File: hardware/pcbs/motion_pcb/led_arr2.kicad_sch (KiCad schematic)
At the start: 21 parts

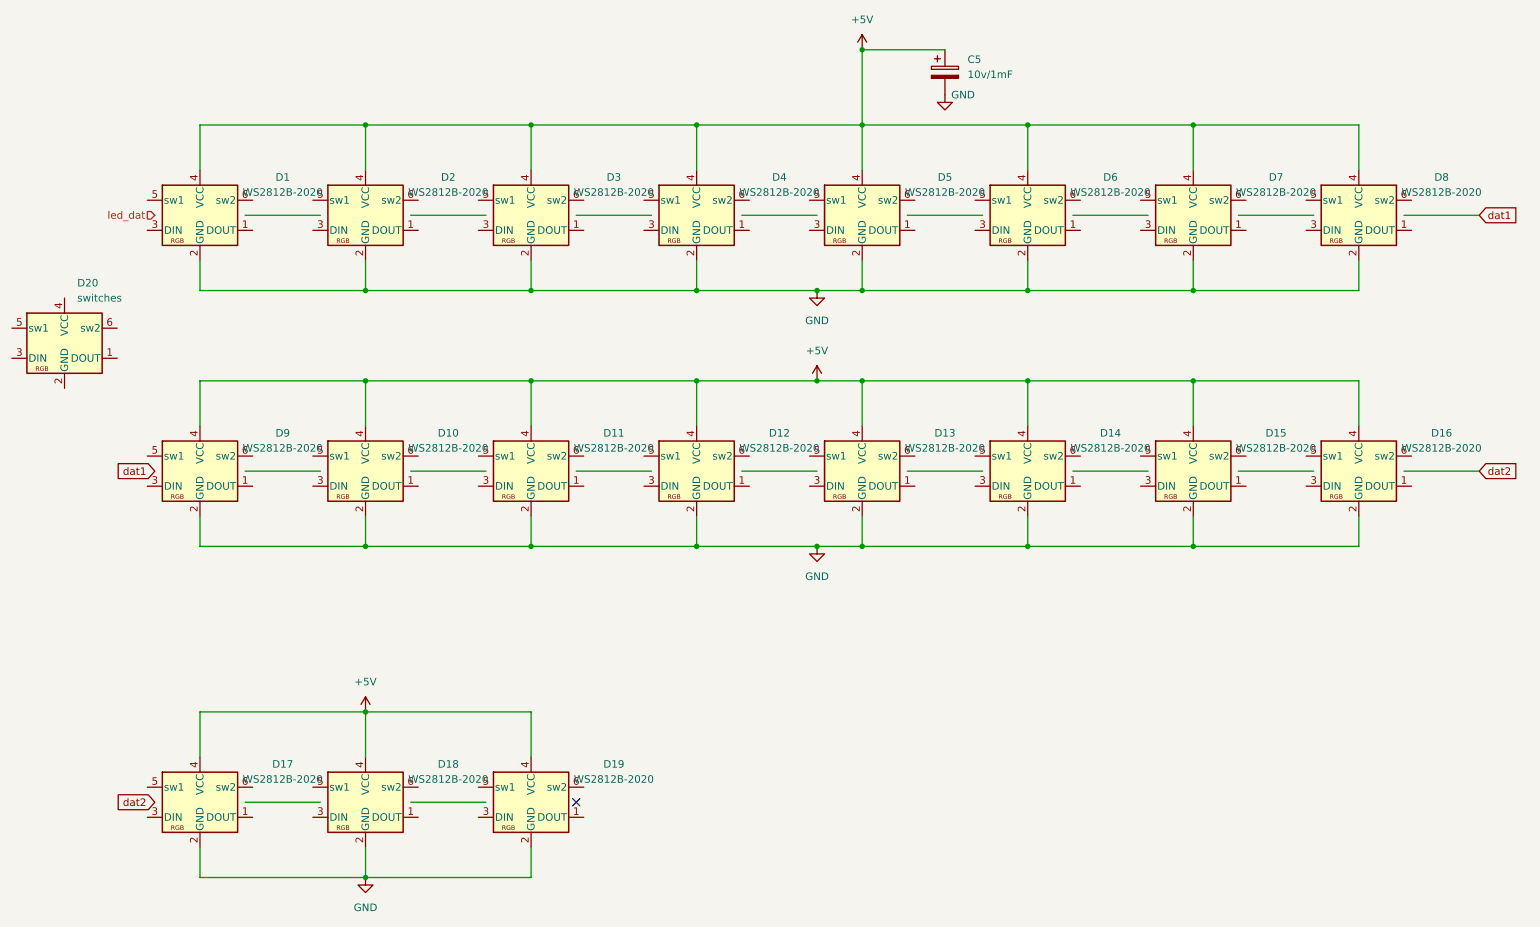
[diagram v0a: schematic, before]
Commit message: finished schematic
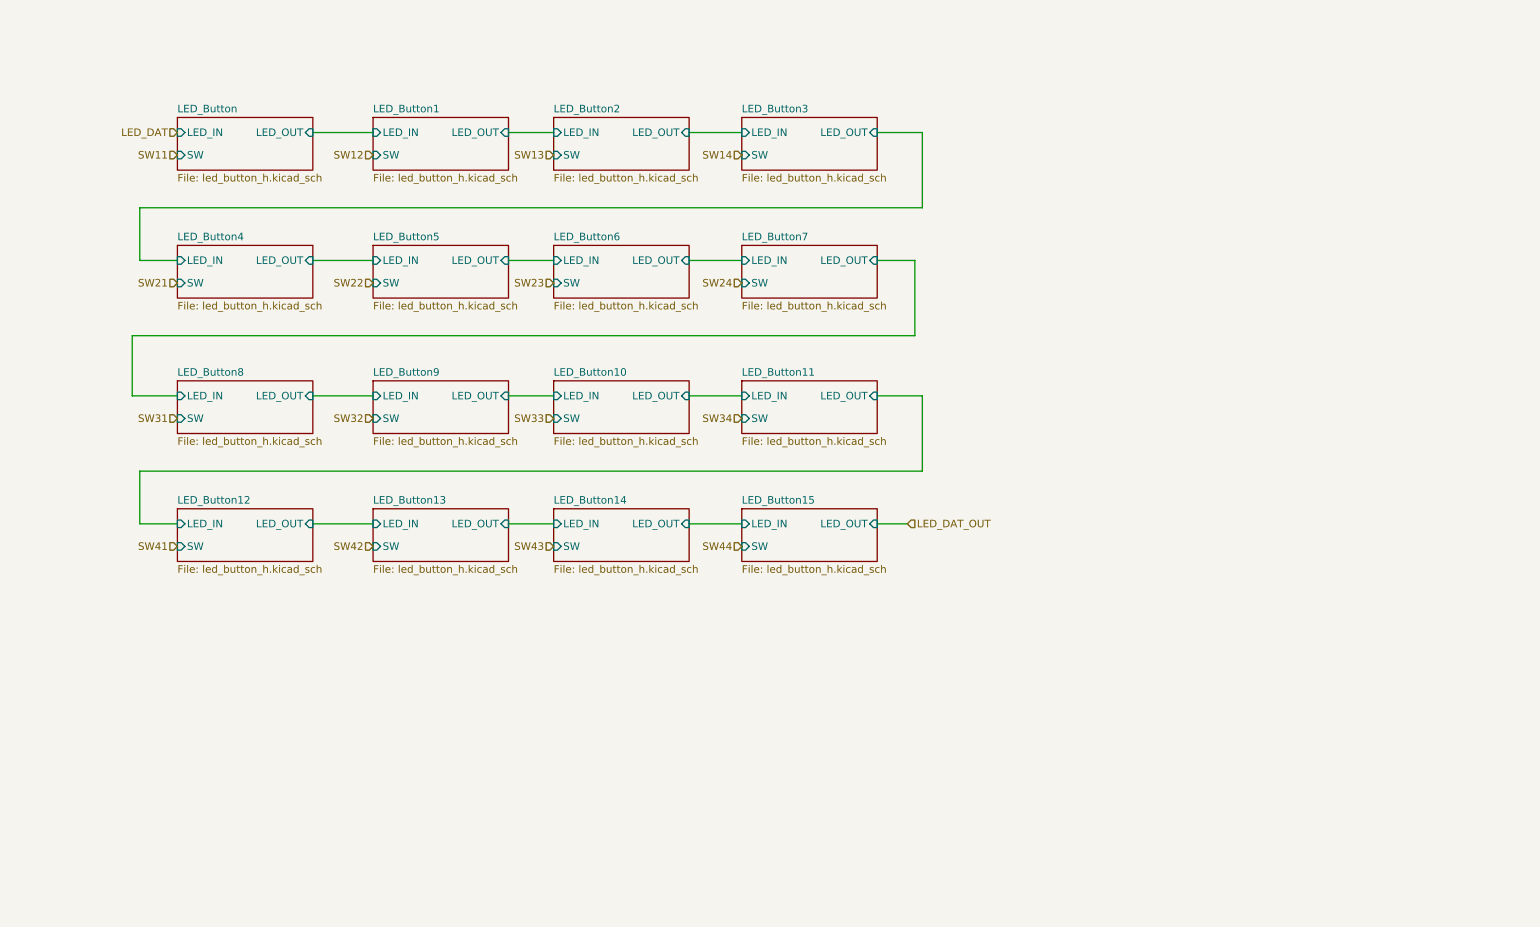
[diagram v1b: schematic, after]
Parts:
- removed C5: 10v/1mF, Capacitor_SMD:CP_Elec_10x10, symbol Device:C_Polarized
- removed D1, D10, D11, D12, D13, D14, D15, D16, D17, D18, D19, D2, D3, D4, D5, D6, D7, D8, D9: WS2812B-2020, LED_SMD:LED_WS2812B-2020_PLCC4_2.0x2.0mm, symbol 3dAudioSym:A3_switches_led
- removed D20: switches, 3dAudioFoot:A3_CherryMxHybrid_WS2812Led2020, symbol 3dAudioSym:A3_switches_led
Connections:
- no-connect marks 1 -> 0
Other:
- added sheet LED_Button (led_button_h.kicad_sch)
- added sheet LED_Button1 (led_button_h.kicad_sch)
- added sheet LED_Button10 (led_button_h.kicad_sch)
- added sheet LED_Button11 (led_button_h.kicad_sch)
- added sheet LED_Button12 (led_button_h.kicad_sch)
- added sheet LED_Button13 (led_button_h.kicad_sch)
- added sheet LED_Button14 (led_button_h.kicad_sch)
- added sheet LED_Button15 (led_button_h.kicad_sch)
- added sheet LED_Button2 (led_button_h.kicad_sch)
- added sheet LED_Button3 (led_button_h.kicad_sch)
- added sheet LED_Button4 (led_button_h.kicad_sch)
- added sheet LED_Button5 (led_button_h.kicad_sch)
- added sheet LED_Button6 (led_button_h.kicad_sch)
- added sheet LED_Button7 (led_button_h.kicad_sch)
- added sheet LED_Button8 (led_button_h.kicad_sch)
- added sheet LED_Button9 (led_button_h.kicad_sch)
